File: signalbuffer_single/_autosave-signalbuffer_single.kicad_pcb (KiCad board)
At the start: 2 copper layers, 35.6 x 17.8 mm, 13 parts, among them J1 GND in, J2 VDD in, J3 VSS in, J4 Signal gnd, J6 Signal In, J7 Bias In, J9 Signal out, U1 LM318N

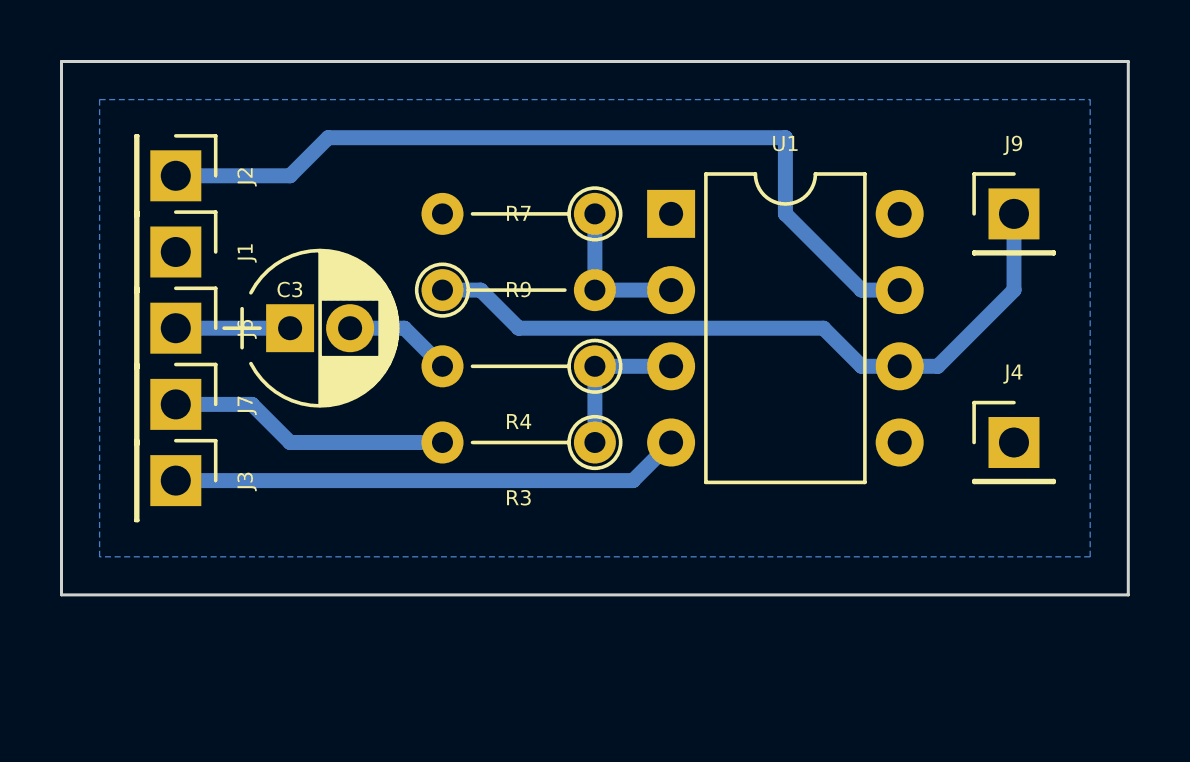
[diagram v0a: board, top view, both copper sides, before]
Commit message: updates
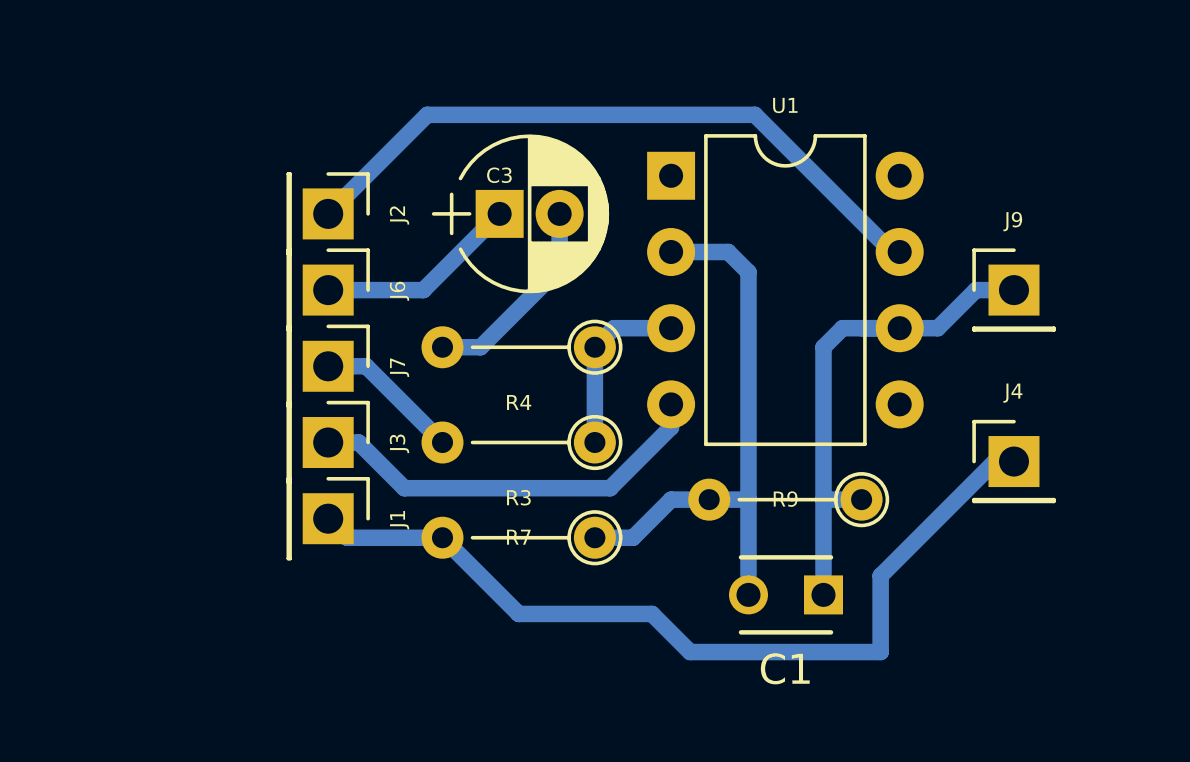
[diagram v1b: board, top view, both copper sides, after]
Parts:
- added C1: C_Small, Capacitors_ThroughHole:C_Disc_D3_P2.5, F.Cu at (160.0, 113.0)
- moved R9 15.6 mm to (161.3, 109.9), turned to 180 degrees
- moved R7 10.8 mm to (152.4, 111.1)
- moved J1 10.2 mm to (143.5, 110.5)
- moved C3 7.96 mm to (149.2, 100.3)
- moved J7 5.24 mm to (143.5, 105.4)
- moved J2 5.24 mm to (143.5, 100.3)
- moved J3 5.24 mm to (143.5, 108.0)
- moved J6 5.24 mm to (143.5, 102.9)
- moved J9 2.54 mm to (166.4, 102.9)
- moved U1 1.27 mm to (154.9, 99.1)
- moved J4 0.63 mm to (166.4, 108.6)
- moved R4 0.63 mm to (152.4, 104.8)
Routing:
- net GNDPWR: track 0.00 -> 28.8 mm
- net Net-(C1-Pad2): track 5.08 -> 19.3 mm
- net Net-(C1-Pad1): track 23.7 -> 17.9 mm
- net Net-(J2-Pad1): track 28.2 -> 22.6 mm
- net Net-(J7-Pad1): track 9.42 -> 4.86 mm
- net Net-(J3-Pad1): track 17.0 -> 13.7 mm
- net Net-(C3-Pad2): track 3.61 -> 6.81 mm
- net Net-(C3-Pad1): track 3.81 -> 6.77 mm
- net Net-(R3-Pad1): track 5.08 -> 5.98 mm
- removed copper zone on B.Cu, net GNDPWR
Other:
- board outline removed
- net class Default: trace_width 0.5 -> 0.55
